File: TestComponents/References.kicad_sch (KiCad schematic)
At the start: 14 parts, among them SW1 SW_DPDT, U13 X, U8 ADR510, U9 LM4040B

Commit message: SpectDrone Development
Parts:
- R4, R5, R9: footprint Capacitor_SMD:C_0805_2012Metric -> Resistor_SMD:R_0805_2012Metric
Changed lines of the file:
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@@
     (property "Reference" "R4" (id 0) (at 126.365 86.36 90))
     (property "Value" "402" (id 1) (at 126.365 90.17 90))
-    (property "Footprint" "Capacitor_SMD:C_0805_2012Metric" (id 2) (at 126.365 91.948 90)
+    (property "Footprint" "Resistor_SMD:R_0805_2012Metric" (id 2) (at 126.365 91.948 90)
       (effects (font (size 1.27 1.27)) hide)
     )
@@
     (property "Reference" "R5" (id 0) (at 126.365 102.235 90))
     (property "Value" "200" (id 1) (at 126.365 106.045 90))
-    (property "Footprint" "Capacitor_SMD:C_0805_2012Metric" (id 2) (at 126.365 107.823 90)
+    (property "Footprint" "Resistor_SMD:R_0805_2012Metric" (id 2) (at 126.365 107.823 90)
       (effects (font (size 1.27 1.27)) hide)
     )
@@
     (property "Reference" "R9" (id 0) (at 141.3901 91.44 90))
     (property "Value" "470K" (id 1) (at 141.3901 93.98 90))
-    (property "Footprint" "Capacitor_SMD:C_0805_2012Metric" (id 2) (at 141.3901 95.758 90)
+    (property "Footprint" "Resistor_SMD:R_0805_2012Metric" (id 2) (at 141.3901 95.758 90)
       (effects (font (size 1.27 1.27)) hide)
     )

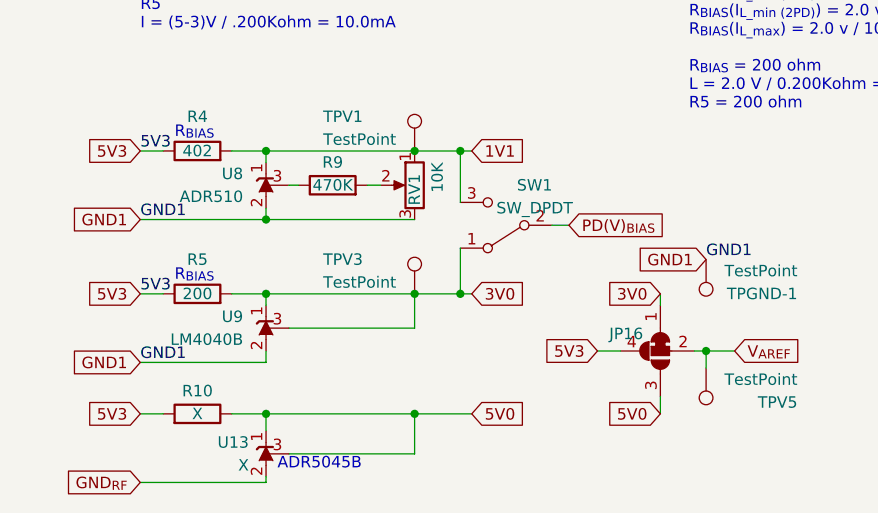
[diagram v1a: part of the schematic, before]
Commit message: SpectDrone Development
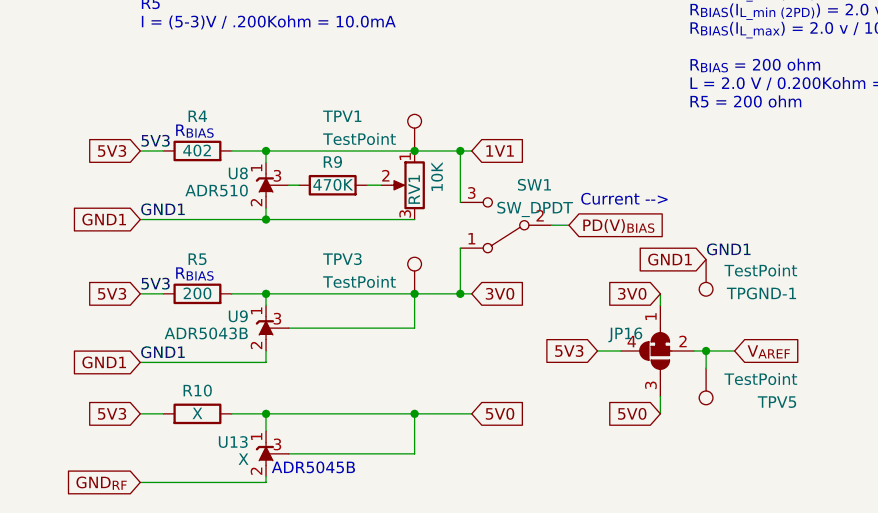
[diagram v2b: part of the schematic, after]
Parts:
- U9: value LM4040B -> ADR5043B
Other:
- note added: "Current -->"
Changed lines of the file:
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@@
     (effects (font (size 1.27 1.27)) (justify left bottom))
   )
-  (text "ADR5045B" (at 135.255 125.73 0)
+  (text "Current -->" (at 168.91 96.52 0)
+    (effects (font (size 1.27 1.27)) (justify left bottom))
+  )
+  (text "ADR5045B" (at 134.62 126.365 0)
     (effects (font (size 1.27 1.27)) (justify left bottom))
   )
@@
   )
   (symbol (lib_name "ADR510_1") (lib_id "Gardenuino_Custom:ADR510") (at 133.985 93.98 270) (mirror x) (unit 1)
-    (in_bom yes) (on_board yes) (fields_autoplaced)
-    (property "Reference" "U8" (id 0) (at 131.445 92.7099 90)
-      (effects (font (size 1.27 1.27)) (justify right))
-    )
-    (property "Value" "ADR510" (id 1) (at 131.445 95.2499 90)
+    (in_bom yes) (on_board yes)
+    (property "Reference" "U8" (id 0) (at 132.08 92.71 90)
+      (effects (font (size 1.27 1.27)) (justify right))
+    )
+    (property "Value" "ADR510" (id 1) (at 132.08 94.615 90)
       (effects (font (size 1.27 1.27)) (justify right))
     )
@@
       (effects (font (size 1.27 1.27)) (justify right))
     )
-    (property "Value" "X" (id 1) (at 132.08 125.095 90)
+    (property "Value" "X" (id 1) (at 132.08 124.46 90)
       (effects (font (size 1.27 1.27)) (justify right))
     )
@@
   (symbol (lib_id "Gardenuino_Custom:ADR510") (at 133.985 109.855 270) (mirror x) (unit 1)
     (in_bom yes) (on_board yes)
-    (property "Reference" "U9" (id 0) (at 131.445 108.585 90)
-      (effects (font (size 1.27 1.27)) (justify right))
-    )
-    (property "Value" "LM4040B" (id 1) (at 131.445 111.125 90)
+    (property "Reference" "U9" (id 0) (at 132.08 108.585 90)
+      (effects (font (size 1.27 1.27)) (justify right))
+    )
+    (property "Value" "ADR5043B" (id 1) (at 132.08 110.49 90)
       (effects (font (size 1.27 1.27)) (justify right))
     )
@@
       (effects (font (size 1.27 1.27) italic) hide)
     )
-    (property "Datasheet" "http://www.cj-elec.com/txUpfile/20134181474991806.pdf" (id 3) (at 133.985 109.855 0)
-      (effects (font (size 1.27 1.27) italic) hide)
-    )
+    (property "Datasheet" "https://www.analog.com/media/en/technical-documentation/data-sheets/ADR5040_5041_5043_5044_5045.pdf" (id 3) (at 133.985 109.855 0)
+      (effects (font (size 1.27 1.27) italic) hide)
+    )

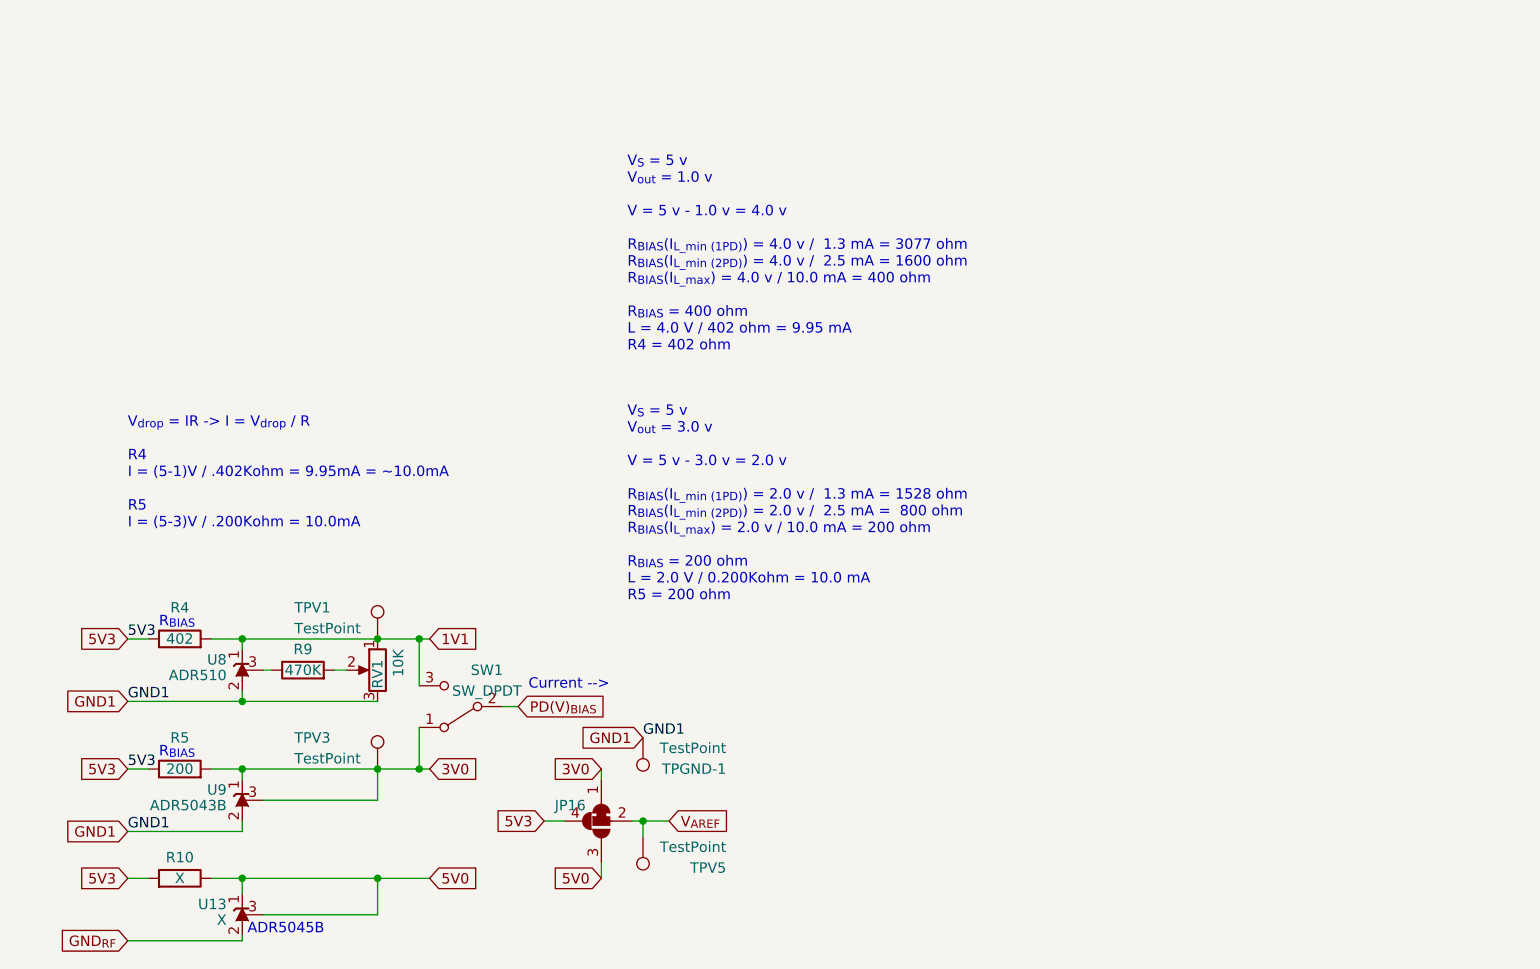
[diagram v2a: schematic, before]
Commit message: SpectDrone Development
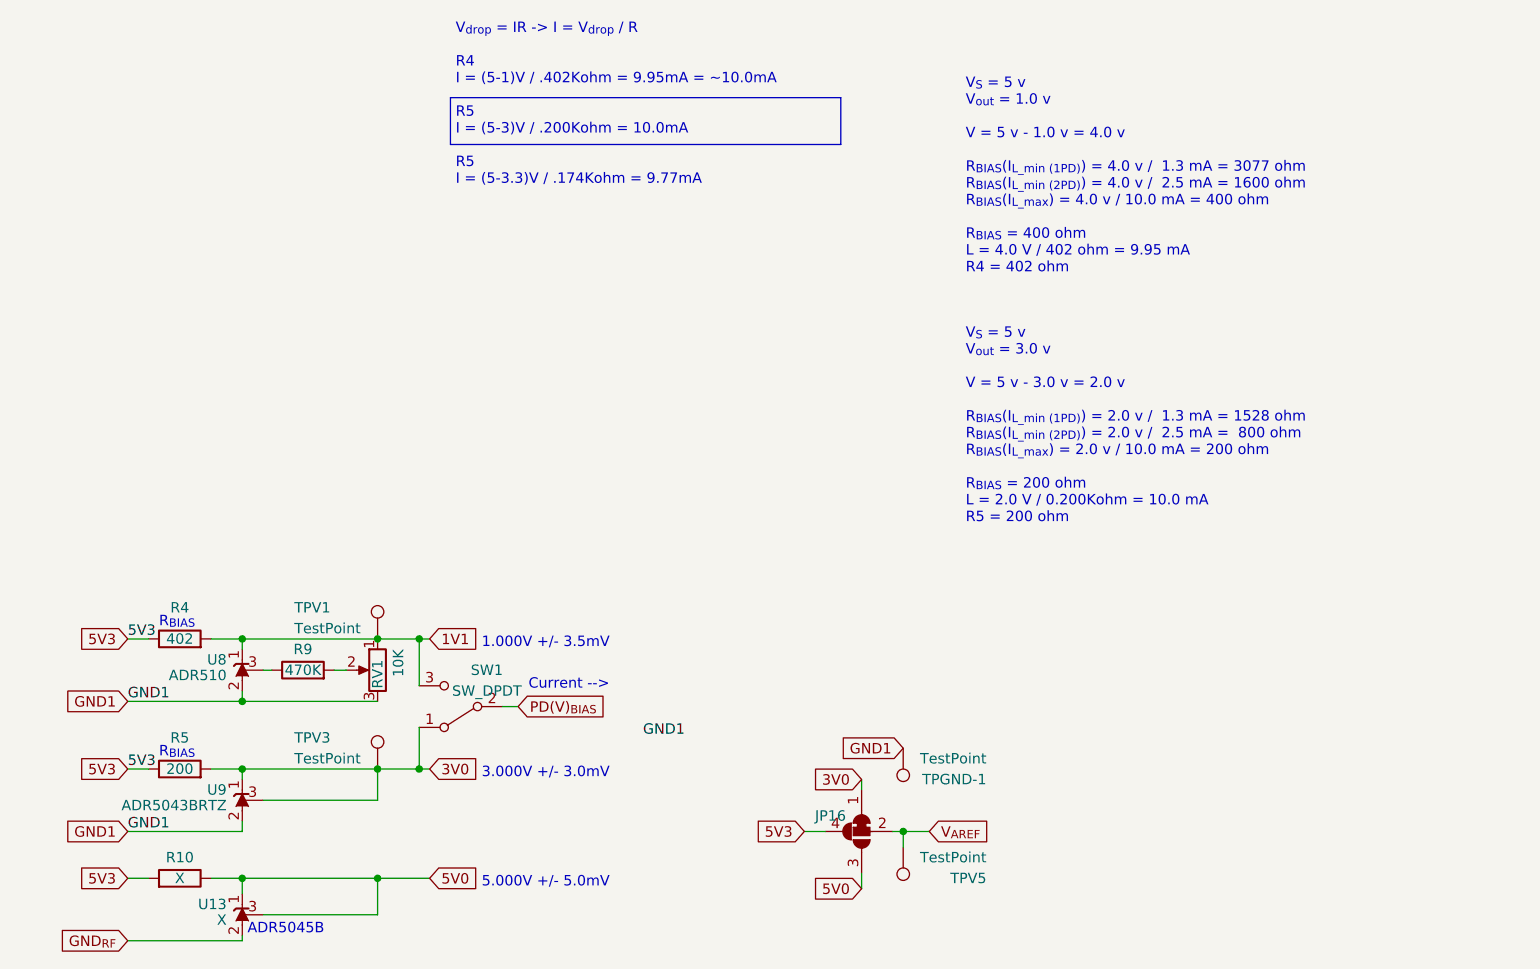
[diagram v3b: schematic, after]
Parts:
- R5: Part Number (none) -> ERJ-6ENF1740V
- U9: value ADR5043B -> ADR5043BRTZ; Part Number (none) -> ADR5043BRTZ
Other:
- note added: "1.000V +/- 3.5mV"
- note added: "3.000V +/- 3.0mV"
- note added: "5.000V +/- 5.0mV"
- note added: "V_{drop} = IR -> I = V_{drop} / R R4 I = (5-1)V / .402Kohm = 9.95mA = ~10.0mA R5 I = (5-3)V / .200Kohm = 10.0mA R5 I = (5-3.3)V / .174Kohm = 9.77mA"
- note removed: "V_{drop} = IR -> I = V_{drop} / R R4 I = (5-1)V / .402Kohm = 9.95mA = ~10.0mA R5 I = (5-3)V / .200Kohm = 10.0mA"
- moved on the sheet: JP16, TPGND-1, TPV5
